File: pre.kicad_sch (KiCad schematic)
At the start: 60 parts, among them J3 Conn_01x03, J4 Conn_01x03, Q1 BSS138, Q2 BSS138, U1 TL072, U2 TL074

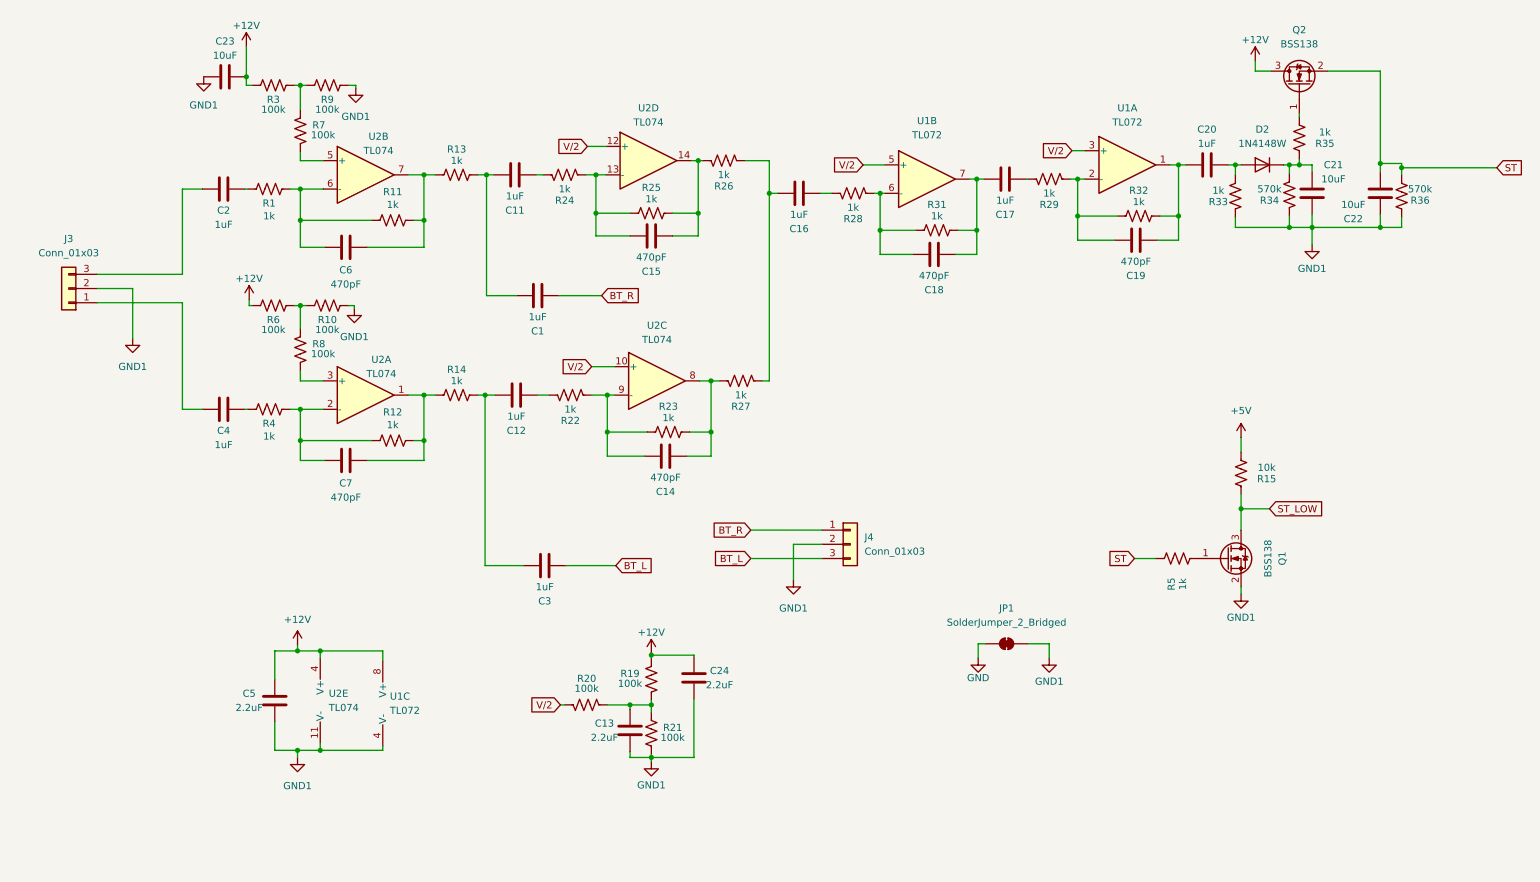
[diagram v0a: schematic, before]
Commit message: v2.0 pre APL_STA2150
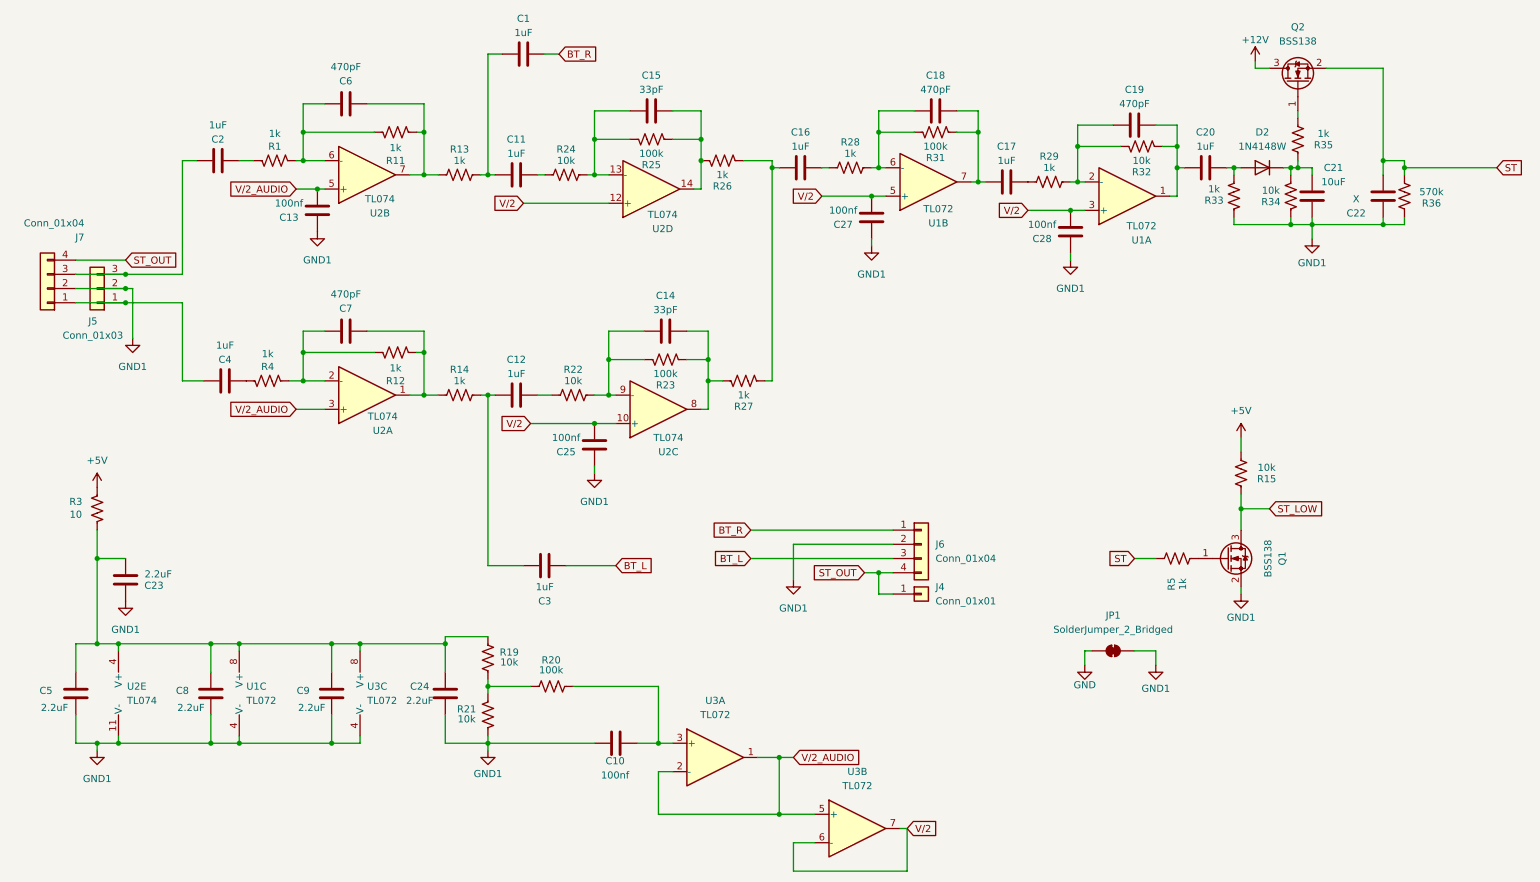
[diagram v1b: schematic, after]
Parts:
- removed J3, J4: Conn_01x03, Connector_JST:JST_XH_B3B-XH-A_1x03_P2.50mm_Vertical, symbol Connector_Generic:Conn_01x03
- removed R10, R6, R7, R8, R9: 100k, Resistor_SMD:R_0805_2012Metric, symbol Device:R_US
- added C10, C25, C27, C28: 100nf, Capacitor_SMD:C_0805_2012Metric, symbol Device:C
- added C8, C9: 2.2uF, Capacitor_SMD:C_0805_2012Metric, symbol Device:C
- added J4: Conn_01x01, Connector_PinHeader_2.54mm:PinHeader_1x01_P2.54mm_Vertical, symbol Connector_Generic:Conn_01x01
- added J5: Conn_01x03, Connector_JST:JST_XH_B3B-XH-A_1x03_P2.50mm_Vertical, symbol Connector_Generic:Conn_01x03
- added J6, J7: Conn_01x04, Connector_JST:JST_XH_B4B-XH-A_1x04_P2.50mm_Vertical, symbol Connector_Generic:Conn_01x04
- added U3: TL072, Package_SO:SOIC-8_3.9x4.9mm_P1.27mm, symbol Amplifier_Operational:TL072
- C13: value 2.2uF -> 100nf
- C14, C15: value 470pF -> 33pF
- C22: value 10uF -> X
- C23: value 10uF -> 2.2uF
- R19, R21: value 100k -> 10k
- R22, R24, R32: value 1k -> 10k
- R23, R25, R31: value 1k -> 100k
- R3: value 100k -> 10
- R34: value 570k -> 10k
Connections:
- net +12V: no longer C23.1, C24.1, C5.1, R19.1, R3.1, U1.8 (V+), U2.4 (V+)
- net +5V: now also R3.1
- net BT_L: now also J6.3 (Pin_3)
- net BT_R: now also C1.1, J6.1 (Pin_1); no longer C1.2
- net GND1: now also C23.1, C10.1, C25.2, C27.2, C28.2, C8.2, C9.2, J5.2 (Pin_2), J6.2 (Pin_2), J7.2 (Pin_2), U3.4 (V-); no longer C23.2
- net V/2: now also C25.1, C27.1, C28.1, U3.6 (-), U3.7; no longer R20.2
- net at R3.2: now also C23.2, C24.1, C5.1, R19.1, U1.8 (V+), U2.4 (V+), C8.1, C9.1, U3.8 (V+)
- net at R19.2, R20.1, R21.1: no longer C13.1
- net V/2_AUDIO: now reaches U2.3 (+)
- net V/2_AUDIO: now also C13.1, U2.5 (+), U3.1, U3.2 (-), U3.5 (+)
- net at C2.2: now also J5.3 (Pin_3), J7.3 (Pin_3)
- net at C11.1, R13.1: now also C1.2; no longer C1.1
- net at C4.2: now also J5.1 (Pin_1), J7.1 (Pin_1)
- new net: C10.2, R20.2, U3.3 (+)
- new net ST_OUT: J4.1 (Pin_1), J6.4 (Pin_4), J7.4 (Pin_4)
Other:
- moved on the sheet: C1, C14, C15, C16, C17, C18, C19, C2, C20, C21, C22, C24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
